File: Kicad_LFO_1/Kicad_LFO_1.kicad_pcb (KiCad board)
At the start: 2 copper layers, 100 x 100 mm, 144 parts, among them J101 LFO555, J102 555 Reset, J103 LFO555Charge, J104 Tri, J105 Sine, J201 In1.1, J202 In1.2, J203 In1.3, J204 Out1, J205 In2, J206 Out2.1, J207 Out2.2, J208 Out2.3, J302 Tri, J303 LFO_SQ, J304 Sine, J401 NAND_IN1, J402 NAND_OUT, J403 NAND_IN2, J404 AND_IN1, J405 AND_OUT, J406 AND_IN2, J407 NOT_OUT, J408 NOT_IN, J501 FF_In1, J502 FF_In2, J503 FF_Out1, J504 FF_Out2, P101 HEADER_2x5_Doepfer, P201 HEADER_2x5_Doepfer, P301 HEADER_2x5_Doepfer, P401 HEADER_2x5_Doepfer, P501 HEADER_2x5_Doepfer, SW101 LFO Low, SW201 Inv/NonInv, SW202 Inv/NonInv, U101 LM555, U102 TL072, U201 TL082, U301 TL072, U302 TL072, U402 74LS00, U501 4013

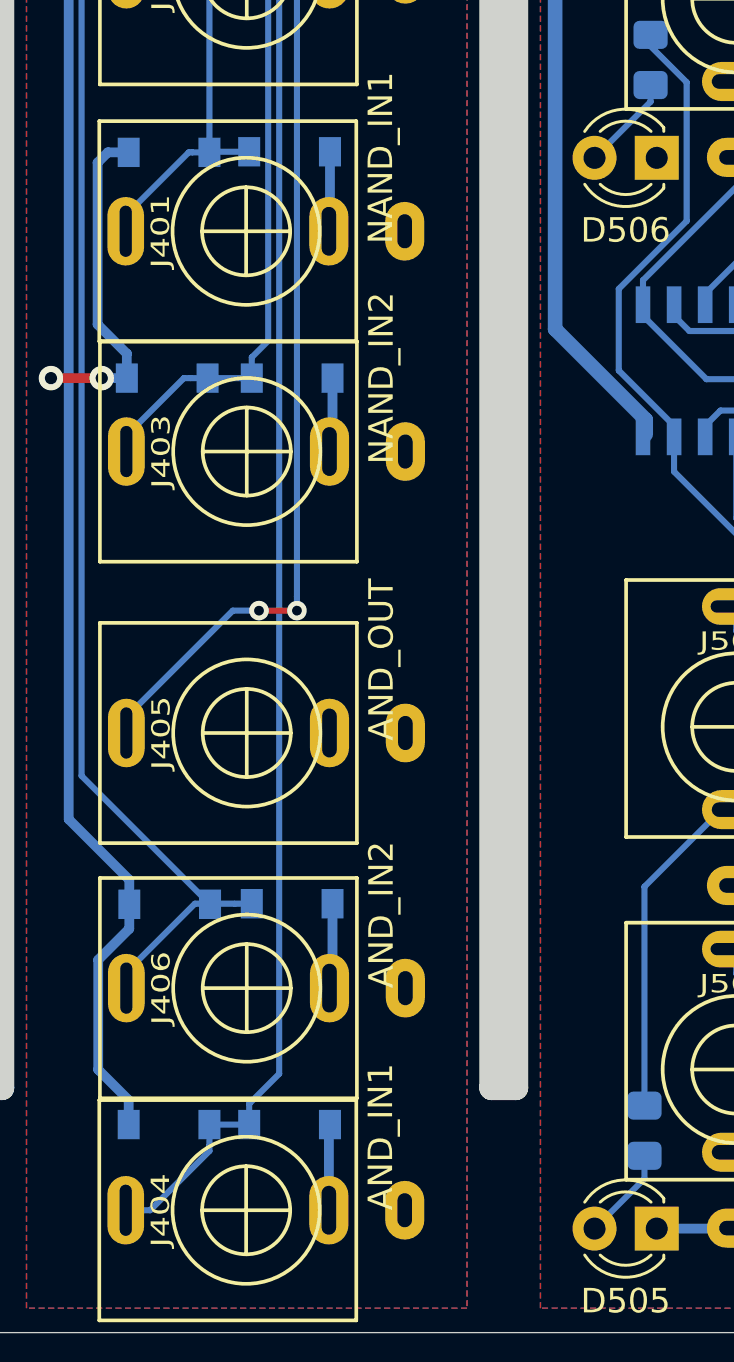
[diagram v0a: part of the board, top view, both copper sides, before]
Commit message: RevB PCB
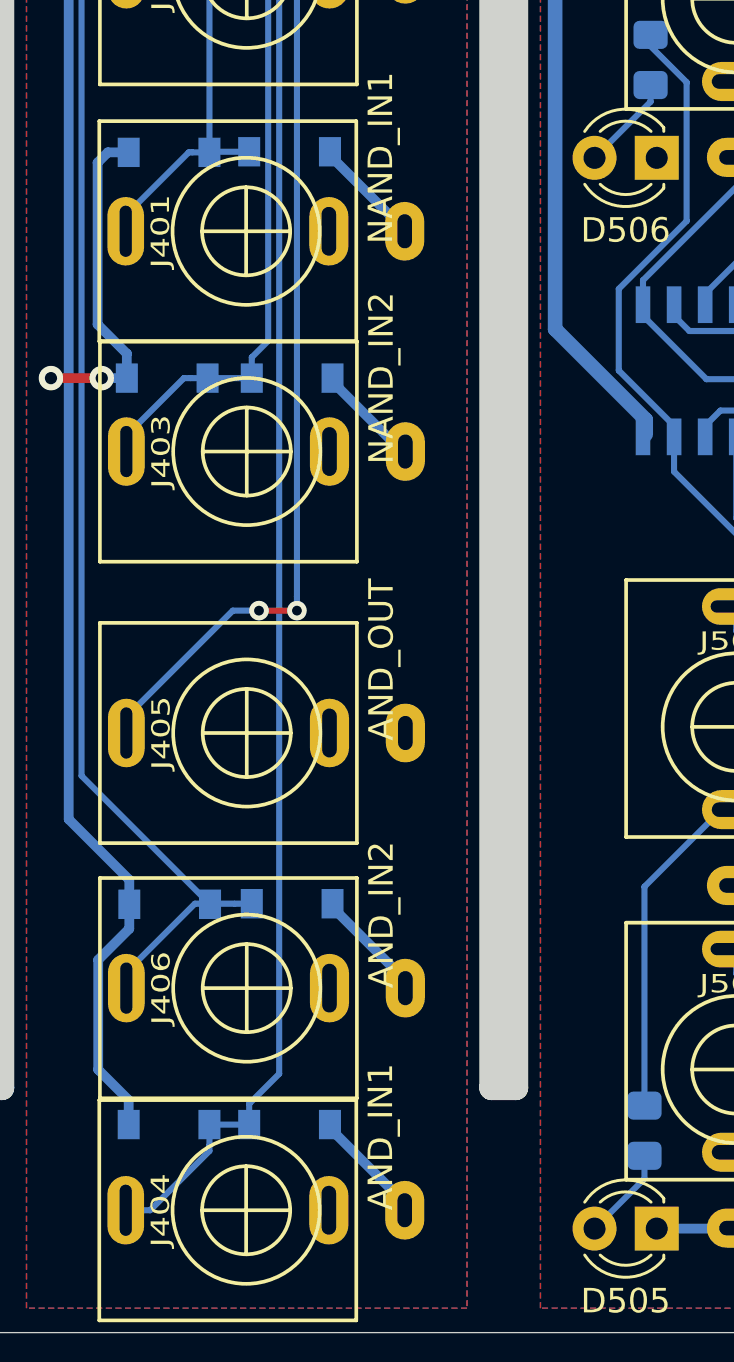
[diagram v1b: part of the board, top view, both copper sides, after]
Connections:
- J401 pad TN: GND -> +12V
- J403 pad TN: GND -> +12V
- J404 pad TN: GND -> +12V
- J406 pad TN: GND -> +12V
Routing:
- net GND: track 301.7 -> 306.6 mm
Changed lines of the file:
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@@
     (thickness 1.6)
     (drawings 38)
-    (tracks 902)
+    (tracks 906)
     (zones 0)
     (modules 144)
@@
       (drillshape 0)
       (scaleselection 1)
-      (outputdirectory "gerber_revA"))
+      (outputdirectory "gerber_revB"))
   )
   (net 0 "")
@@
     (fp_circle (center 0 0) (end 1.8 0) (layer F.SilkS) (width 0.15))
     (pad TN thru_hole oval (at 0 3.38 90) (size 2.8 1.6) (drill oval 2 0.6) (layers *.Cu *.Mask)
-      (net 1 GND))
+      (net 6 +12V))
     (pad S thru_hole oval (at 0 6.48 90) (size 2.4 1.6) (drill oval 1.4 0.6) (layers *.Cu *.Mask)
       (net 1 GND))
@@
       (net 1 GND))
     (pad TN thru_hole oval (at 0 3.38 90) (size 2.8 1.6) (drill oval 2 0.6) (layers *.Cu *.Mask)
-      (net 1 GND))
+      (net 6 +12V))
     (model ${KIPRJMOD}/Local.pretty/PJ398SM.step
       (offset (xyz 0 0 9))
@@
       (net 1 GND))
     (pad TN thru_hole oval (at 0 3.38 90) (size 2.8 1.6) (drill oval 2 0.6) (layers *.Cu *.Mask)
-      (net 1 GND))
+      (net 6 +12V))
     (model ${KIPRJMOD}/Local.pretty/PJ398SM.step
       (offset (xyz 0 0 9))
@@
     (fp_circle (center 0 0) (end 1.8 0) (layer F.SilkS) (width 0.15))
     (pad TN thru_hole oval (at 0 3.38 90) (size 2.8 1.6) (drill oval 2 0.6) (layers *.Cu *.Mask)
-      (net 1 GND))
+      (net 6 +12V))
     (pad S thru_hole oval (at 0 6.48 90) (size 2.4 1.6) (drill oval 1.4 0.6) (layers *.Cu *.Mask)
       (net 1 GND))
@@
   (segment (start 103.4 80.205001) (end 103.355001 80.25) (width 0.4) (layer B.Cu) (net 1))
   (segment (start 103.4 75.5) (end 103.4 80.205001) (width 0.4) (layer B.Cu) (net 1))
-  (segment (start 103.4 104.955001) (end 103.355001 105) (width 0.4) (layer B.Cu) (net 1))
-  (segment (start 103.4 101.75) (end 103.4 104.955001) (width 0.4) (layer B.Cu) (net 1))
-  (segment (start 103.505001 113.874999) (end 103.38 114) (width 0.4) (layer B.Cu) (net 1))
-  (segment (start 103.505001 111) (end 103.505001 113.874999) (width 0.4) (layer B.Cu) (net 1))
-  (segment (start 103.355001 141.544999) (end 103.4 141.5) (width 0.4) (layer B.Cu) (net 1))
-  (segment (start 103.355001 145) (end 103.355001 141.544999) (width 0.4) (layer B.Cu) (net 1))
-  (segment (start 103.505001 135.799998) (end 103.38 135.924999) (width 0.4) (layer B.Cu) (net 1))
-  (segment (start 103.505001 132.474999) (end 103.505001 135.799998) (width 0.4) (layer B.Cu) (net 1))
   (via (at 95 83) (size 1) (drill 0.5) (layers F.Cu B.Cu) (net 1))
   (segment (start 97.05 83.44) (end 95.44 83.44) (width 0.4) (layer B.Cu) (net 1))
@@
   (via (at 132.5 108.75) (size 1) (drill 0.5) (layers F.Cu B.Cu) (net 1))
   (segment (start 132.8 108.75) (end 132.5 108.75) (width 0.4) (layer B.Cu) (net 1))
+  (segment (start 106.455001 104.955001) (end 106.455001 105) (width 0.4) (layer B.Cu) (net 1))
+  (segment (start 103.4 101.9) (end 106.455001 104.955001) (width 0.4) (layer B.Cu) (net 1))
+  (segment (start 103.4 101.75) (end 103.4 101.9) (width 0.4) (layer B.Cu) (net 1))
+  (segment (start 106.355001 114) (end 106.48 114) (width 0.4) (layer B.Cu) (net 1))
+  (segment (start 103.505001 111.15) (end 106.355001 114) (width 0.4) (layer B.Cu) (net 1))
+  (segment (start 103.505001 111) (end 103.505001 111.15) (width 0.4) (layer B.Cu) (net 1))
+  (segment (start 106.48 135.599998) (end 106.48 135.924999) (width 0.4) (layer B.Cu) (net 1))
+  (segment (start 103.505001 132.624999) (end 106.48 135.599998) (width 0.4) (layer B.Cu) (net 1))
+  (segment (start 103.505001 132.474999) (end 103.505001 132.624999) (width 0.4) (layer B.Cu) (net 1))
+  (segment (start 106.455001 144.705001) (end 106.455001 145) (width 0.4) (layer B.Cu) (net 1))
+  (segment (start 103.4 141.65) (end 106.455001 144.705001) (width 0.4) (layer B.Cu) (net 1))
+  (segment (start 103.4 141.5) (end 103.4 141.65) (width 0.4) (layer B.Cu) (net 1))
   (segment (start 62.595 66.62) (end 62.5 66.525) (width 0.25) (layer B.Cu) (net 2))
   (segment (start 62.595 69.2) (end 62.595 66.62) (width 0.25) (layer B.Cu) (net 2))
